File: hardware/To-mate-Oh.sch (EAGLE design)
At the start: 25 parts, among them IC1 Tiny45-20-SMT

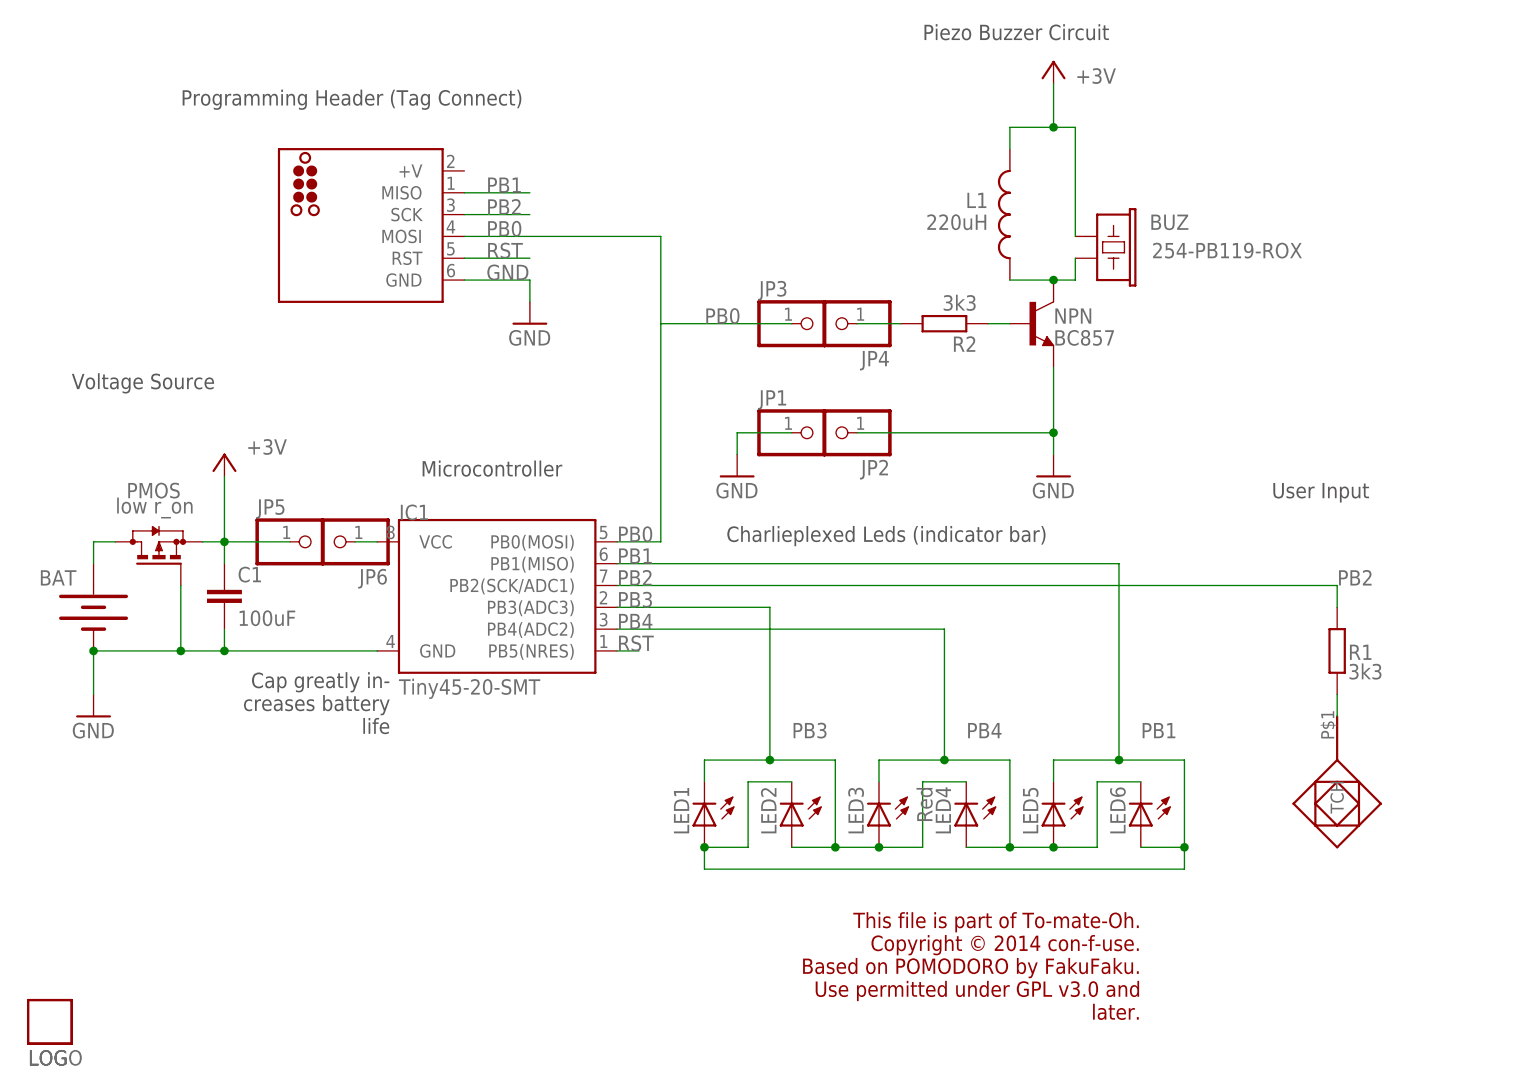
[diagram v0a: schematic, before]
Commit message: Added readme
Update README.md

Update README.md

Update README.md

Update README.md

Update README.md

Minor cosmetics

Minor cosmetics

Minor cosmetics

Update README.md
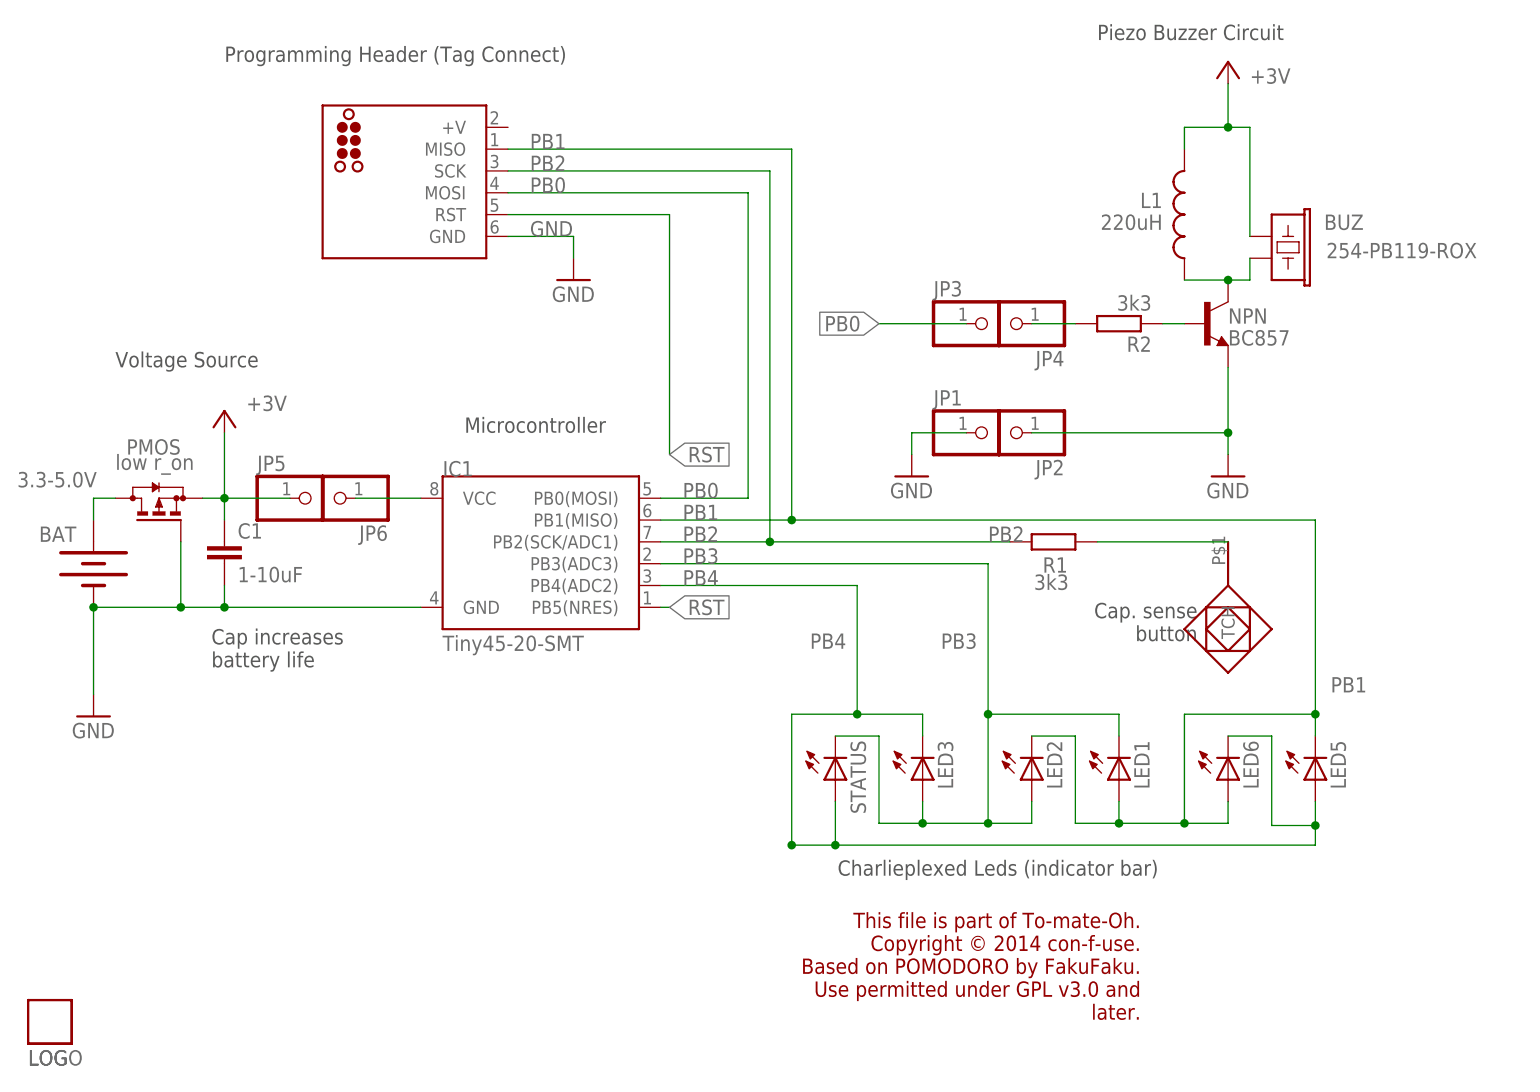
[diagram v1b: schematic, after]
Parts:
- removed LED4: Red, led:LEDCHIPLED_0805
- removed U$1: PAD, jcgb:PAD
- added CAP_SENSE: PAD, jcgb:PAD
- added STATUS: Red, led:LEDCHIPLED_0805
- BAT: value (none) -> 3.3-5.0V
- C1: value 100uF -> 1-10uF
- JP1: value (none) -> JGND1
- JP2: value (none) -> JGND2
- JP3: value (none) -> JPB1
- JP4: value (none) -> JPB2
- JP5: value (none) -> JVCC1
- JP6: value (none) -> JVCC2
- LED1, LED2, LED3, LED5, LED6: value (none) -> Blue
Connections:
- net VBAT renamed BAT+
- net BTN: now also CAP_SENSE.TCH; no longer U$1.TCH
- net PB3: now also STATUS.C; no longer LED4.C
- net PB4: now also STATUS.A; no longer LED4.A
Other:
- note added: "Cap increases battery life"
- note added: "Cap. sense button"
- note removed: "Cap greatly in- creases battery life"
- note removed: "User Input"
- moved on the sheet: BAT, BUZ, C1, IC1, JP1, JP2, JP3, JP4, JP5, JP6, L1, LED1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
